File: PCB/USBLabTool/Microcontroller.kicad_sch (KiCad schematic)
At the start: 15 parts, among them SW2 PTH_RA_h7.5mm, U12 STM32H562VGTx, Y1 32.768kHz

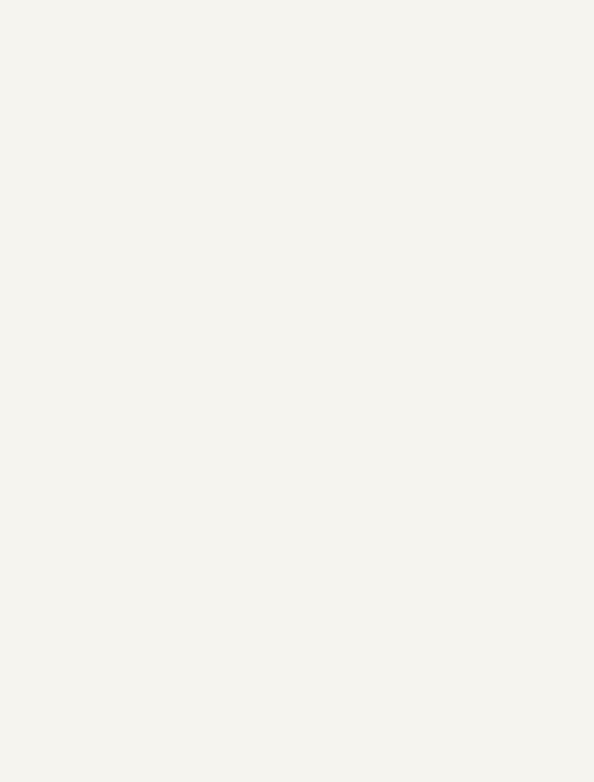
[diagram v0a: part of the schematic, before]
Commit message: Started adding 20pin
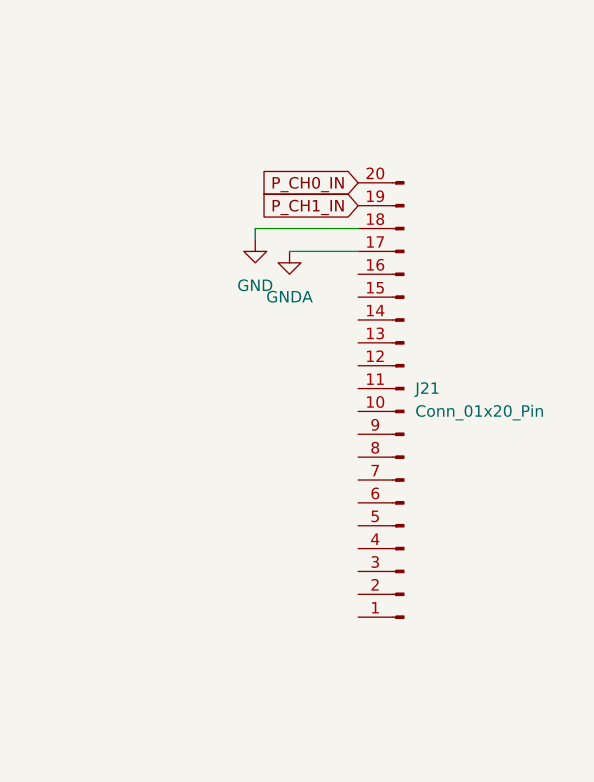
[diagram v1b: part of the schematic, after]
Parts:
- added J21: Conn_01x20_Pin, Connector_PinHeader_2.54mm:PinHeader_1x20_P2.54mm_Vertical, symbol Connector:Conn_01x20_Pin
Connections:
- net GND: now also J21.18 (Pin_18)
- net GNDA: now also J21.17 (Pin_17)
- new net P_CH0_IN: J21.20 (Pin_20)
- new net P_CH1_IN: J21.19 (Pin_19)
